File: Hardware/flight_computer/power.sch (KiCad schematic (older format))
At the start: 49 parts, among them Q3 PMOS_20V_.76A, U6 Buck_Converter_2, U7 LDO_600MA, U8 LP5907QMFX-3.3, U9 LP5907QMFX-3.3

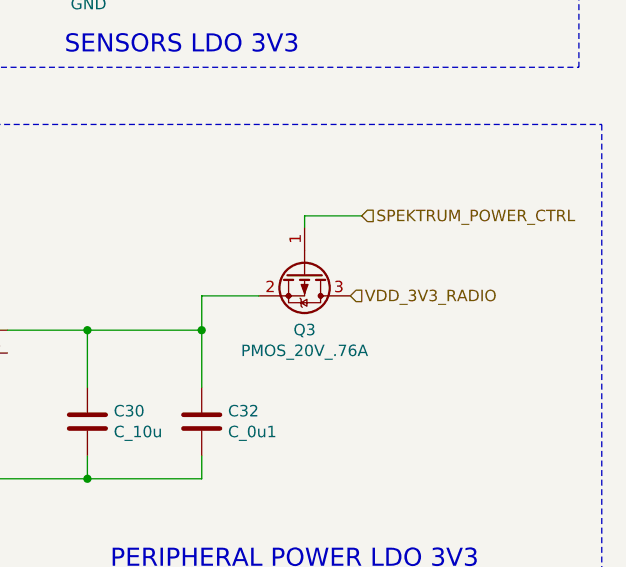
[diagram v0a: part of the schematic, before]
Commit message: worked on layout
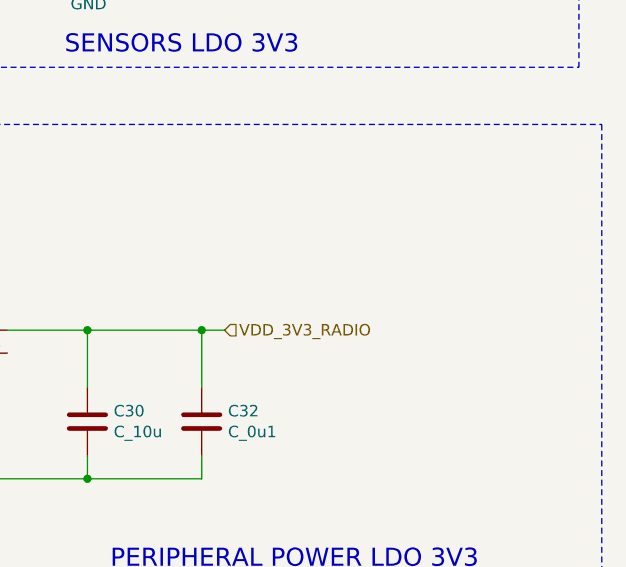
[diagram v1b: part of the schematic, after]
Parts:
- removed Q3: PMOS_20V_.76A, drone_footprints:NTA4151PT1G, symbol openDrone_parts:PMOS_20V_.76A
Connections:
- net VDD_3V3_RADIO: now also C30.1, C32.1, U7.5 (VO)
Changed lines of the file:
@@
 Wire Wire Line
 	13550 5300 14050 5300
-Text HLabel 14750 4800 2    50   Input ~ 0
-SPEKTRUM_POWER_CTRL
-Wire Wire Line
-	14750 4800 14500 4800
-Wire Wire Line
-	14500 4800 14500 4850
-Wire Wire Line
-	14300 5150 14050 5150
-Wire Wire Line
-	14050 5150 14050 5300
-Connection ~ 14050 5300
-Text HLabel 14700 5150 2    50   Input ~ 0
+Text HLabel 14150 5300 2    50   Input ~ 0
 VDD_3V3_RADIO
 Text Notes 14850 2650 0    79   ~ 0
@@
 	14500 1250 14900 1250
 $Comp
-L openDrone_parts:PMOS_20V_.76A Q3
-U 1 1 5FAD41DB
-P 14500 5050
-F 0 "Q3" V 14749 5050 50  0000 C CNN
-F 1 "PMOS_20V_.76A" V 14840 5050 50  0000 C CNN
-F 2 "drone_footprints:NTA4151PT1G" H 13950 5350 50  0001 C CNN
-F 3 "" H 14500 5050 50  0001 C CNN
-F 4 "NTA4151PT1GOSCT-ND" H 14000 5250 50  0001 C CNN "DPN"
-F 5 "NTA4151PT1G" H 13850 5150 50  0001 C CNN "MPN"
-	1    14500 5050
-	0    1    1    0
-$EndComp
-$Comp
 L openDrone_parts:PTC_6V_2A F1
 U 1 1 5FB0D3CF
@@
 	4300 1250 4300 1150
 Connection ~ 4300 1150
+Connection ~ 14050 5300
+Wire Wire Line
+	14050 5300 14150 5300
 $EndSCHEMATC
